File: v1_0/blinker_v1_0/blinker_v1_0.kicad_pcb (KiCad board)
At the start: 2 copper layers, 23 parts, among them J3 Barrel_Jack_Switch_Pin3Ring, Q1 2N7002K, SW1 SW_DIP_x02, SW2 SW_DIP_x02, U1 NE555D, U2 LM1117MP-ADJ

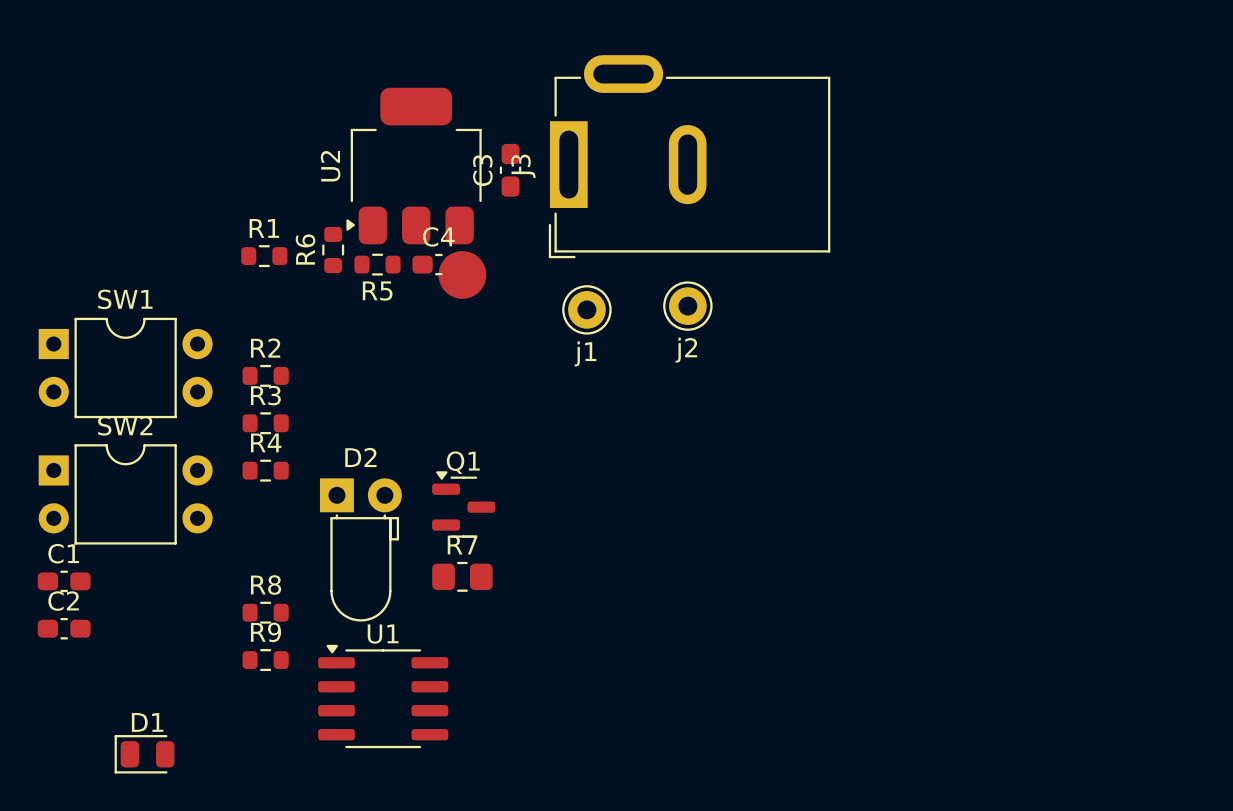
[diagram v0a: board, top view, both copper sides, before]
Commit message: lyt cont, outline is developing
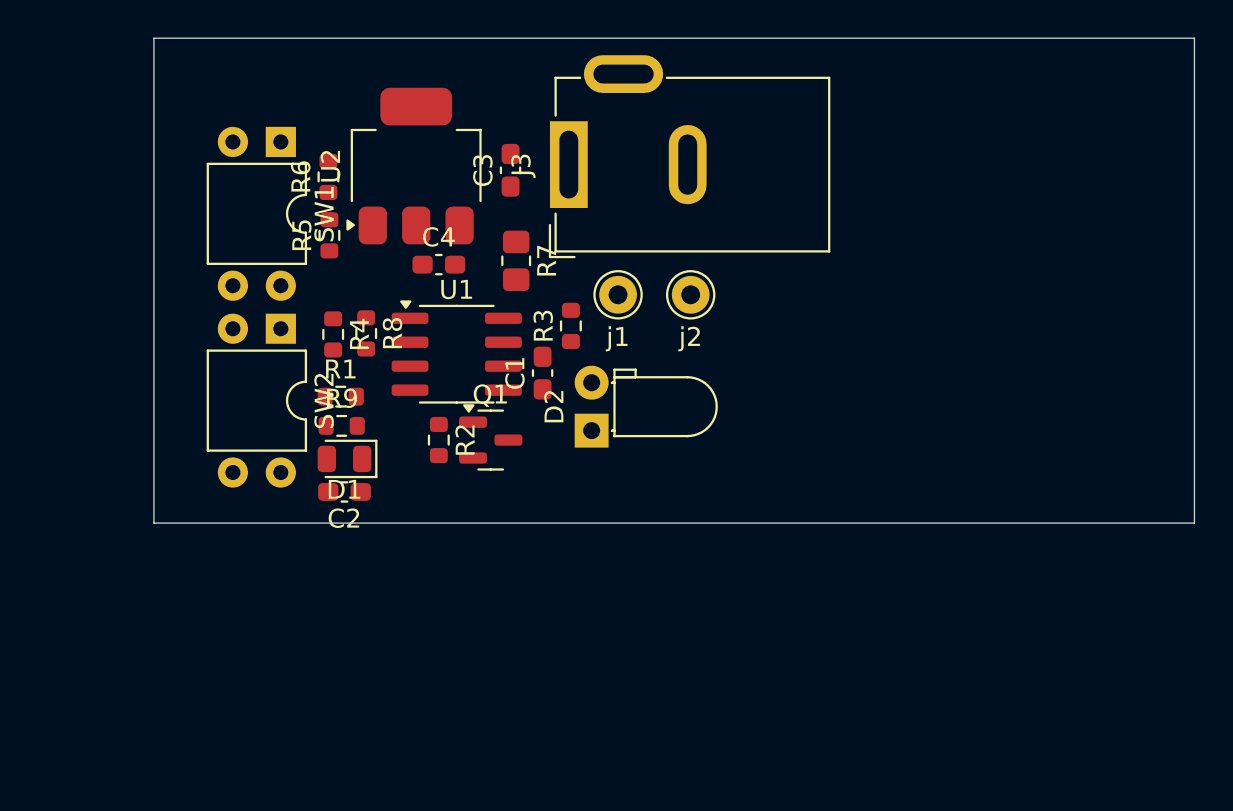
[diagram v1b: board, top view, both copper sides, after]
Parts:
- moved C1 27.7 mm to (166.2, 45.7), turned to 90 degrees
- moved D1 18.8 mm to (155.8, 50.2), turned to 180 degrees
- moved U1 18.7 mm to (161.7, 44.7)
- moved R7 17.0 mm to (164.8, 39.8), turned to -90 degrees
- moved R3 17.0 mm to (167.8, 43.2), turned to 90 degrees
- moved C2 16.5 mm to (155.8, 52.0), turned to 180 degrees
- moved SW1 16.1 mm to (152.4, 33.5), turned to -90 degrees
- moved R8 15.7 mm to (156.9, 43.6), turned to -90 degrees
- moved SW2 14.2 mm to (152.4, 43.4), turned to -90 degrees
- moved D2 13.9 mm to (168.8, 48.8), turned to 90 degrees
- moved R9 13.0 mm to (155.6, 48.5)
- moved R2 9.79 mm to (160.8, 49.2), turned to -90 degrees
- moved R1 8.48 mm to (155.6, 47.0)
- moved R4 8.06 mm to (155.2, 43.6), turned to -90 degrees
- moved R6 3.88 mm to (154.9, 35.3)
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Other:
- board outline added: 55.2 x 25.7 mm
